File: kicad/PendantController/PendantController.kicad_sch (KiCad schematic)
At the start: 27 parts, among them J1 RotaryEncoder, J10 Btn7, J11 Btn8, J2 Switches, J3 DC24V, J4 Btn1, J5 Btn2, J6 Btn3, J7 Btn4, J8 Btn5, J9 Btn6, U1 Arduino_Micro, U2 ULN2803A

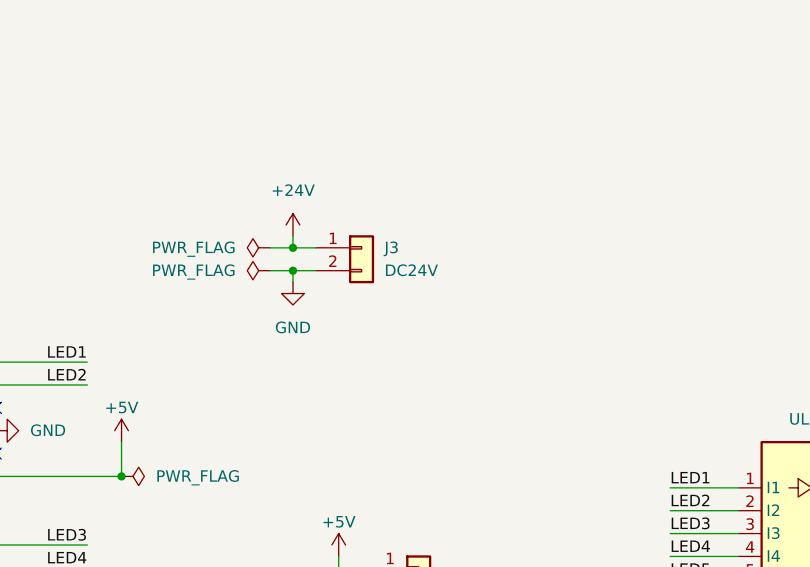
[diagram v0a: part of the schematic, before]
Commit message: Updated PCB layout
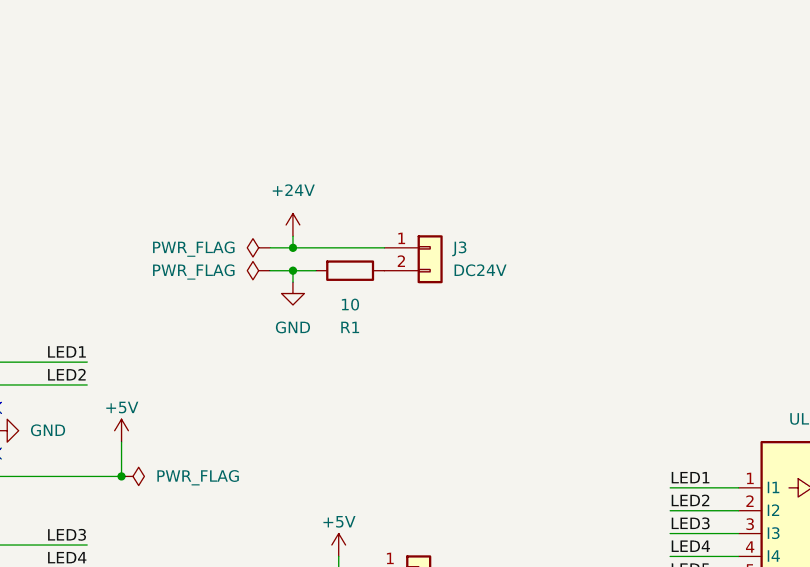
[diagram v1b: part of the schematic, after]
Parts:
- added R1: 10, Resistor_THT:R_Axial_DIN0309_L9.0mm_D3.2mm_P12.70mm_Horizontal, symbol Device:R
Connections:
- net GND: now also R1.2; no longer J3.2 (Pin_2)
- new net: J3.2 (Pin_2), R1.1
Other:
- moved on the sheet: J3
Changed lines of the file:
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@@
 	(wire
 		(pts
-			(xy 128.27 45.72) (xy 130.81 45.72)
+			(xy 128.27 45.72) (xy 138.43 45.72)
 		)
 		(stroke
@@
 	(symbol
 		(lib_id "Connector_Generic:Conn_01x02")
-		(at 135.89 45.72 0)
+		(at 143.51 45.72 0)
 		(unit 1)
 		(exclude_from_sim no)
@@
 		(fields_autoplaced yes)
 		(property "Reference" "J3"
-			(at 138.43 45.7199 0)
+			(at 146.05 45.7199 0)
 			(effects
 				(font
@@
 		)
 		(property "Value" "DC24V"
-			(at 138.43 48.2599 0)
+			(at 146.05 48.2599 0)
 			(effects
 				(font
@@
 		)
 		(property "Footprint" "Connector_PinHeader_2.54mm:PinHeader_1x02_P2.54mm_Vertical"
-			(at 135.89 45.72 0)
+			(at 143.51 45.72 0)
 			(effects
 				(font
@@
 		)
 		(property "Datasheet" "~"
-			(at 135.89 45.72 0)
+			(at 143.51 45.72 0)
 			(effects
 				(font
@@
 		)
 		(property "Description" "Generic connector, single row, 01x02, script generated (kicad-library-utils/schlib/autogen/connector/)"
-			(at 135.89 45.72 0)
+			(at 143.51 45.72 0)
 			(effects
 				(font
@@
 					(unit 1)
 				)
+			)
+		)
+	)
+	(symbol
+		(lib_id "Device:R")
+		(at 134.62 48.26 270)
+		(unit 1)
+		(exclude_from_sim no)
+		(in_bom yes)
+		(on_board yes)
+		(dnp no)
+		(property "Reference" "R1"
+			(at 134.62 54.61 90)
+			(effects
+				(font
+					(size 1.27 1.27)
+				)
+			)
+		)
+		(property "Value" "10"
+			(at 134.62 52.07 90)
+			(effects
+				(font
+					(size 1.27 1.27)
+				)
+			)
+		)
+		(property "Footprint" "Resistor_THT:R_Axial_DIN0309_L9.0mm_D3.2mm_P12.70mm_Horizontal"
+			(at 134.62 46.482 90)
+			(effects
+				(font
+					(size 1.27 1.27)
+				)
+				(hide yes)
+			)
+		)
+		(property "Datasheet" "~"
+			(at 134.62 48.26 0)
+			(effects
+				(font
+					(size 1.27 1.27)
+				)
+				(hide yes)
+			)
+		)
+		(property "Description" "Resistor"
+			(at 134.62 48.26 0)
+			(effects
+				(font
+					(size 1.27 1.27)
+				)
+				(hide yes)
+			)
+		)
+		(pin "1"
+		)
+		(pin "2"
+		)
+		(instances
+			(project "PendantController"
+				(path "/97d16841-8b77-4c29-a79d-2680519e8080"
+					(reference "R1")
+					(unit 1)
+				)
